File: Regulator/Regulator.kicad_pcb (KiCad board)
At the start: 2 copper layers, 10.2 x 12.7 mm, 10 parts, among them J1 Conn_01x04, U1 LMR16006+FB

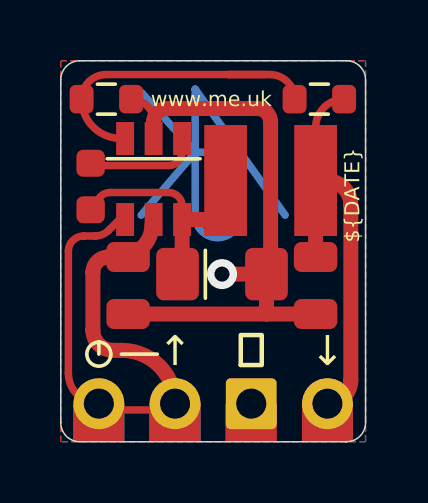
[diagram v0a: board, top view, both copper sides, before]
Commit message: Tweak
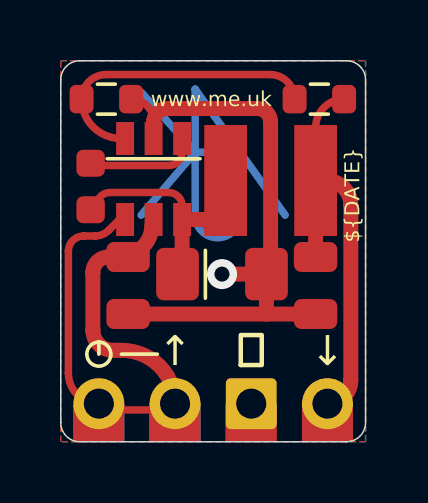
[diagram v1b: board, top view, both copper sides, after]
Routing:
- net Net-(R1-Pad2): track 11.4 -> 10.1 mm
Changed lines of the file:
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@@
   (segment (start 166.33404 62.412) (end 165.9755 62.412) (width 0.5) (layer "F.Cu") (net 2))
   (segment (start 167.15002 69.06998) (end 167.15002 63.22798) (width 0.5) (layer "F.Cu") (net 2))
-  (arc (start 166.1485 61.994342) (mid 166.103539 62.220377) (end 165.9755 62.412) (width 0.5) (layer "F.Cu") (net 2))
   (arc (start 167.15002 63.22798) (mid 166.911025 62.650995) (end 166.33404 62.412) (width 0.5) (layer "F.Cu") (net 2))
   (arc (start 166.925 59.7) (mid 166.253602 59.978102) (end 165.9755 60.6495) (width 0.25) (layer "F.Cu") (net 2))
   (arc (start 166.37 69.85) (mid 166.921557 69.621537) (end 167.15002 69.06998) (width 0.5) (layer "F.Cu") (net 2))
-  (segment (start 164.33398 58.87948) (end 163.07948 58.87948) (width 0.25) (layer "F.Cu") (net 3))
   (segment (start 159.487 61.012) (end 159.6255 61.012) (width 0.25) (layer "F.Cu") (net 3))
-  (segment (start 163.07948 58.87948) (end 158.99552 58.87948) (width 0.25) (layer "F.Cu") (net 3))
-  (segment (start 163.07948 58.87948) (end 164.45448 58.87948) (width 0.25) (layer "F.Cu") (net 3))
+  (segment (start 158.99552 58.87948) (end 164.45448 58.87948) (width 0.25) (layer "F.Cu") (net 3))
   (arc (start 158.175 59.7) (mid 158.559276 60.627724) (end 159.487 61.012) (width 0.25) (layer "F.Cu") (net 3))
   (arc (start 164.45448 58.87948) (mid 165.034675 59.119805) (end 165.275 59.7) (width 0.25) (layer "F.Cu") (net 3))

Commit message: Tweaks
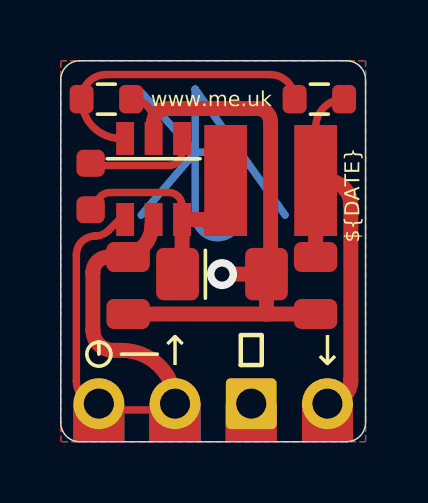
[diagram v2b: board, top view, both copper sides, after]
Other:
- rule pad_to_mask_clearance: 0 -> 0.125
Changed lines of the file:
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@@
       (dielectric_constraints no)
     )
-    (pad_to_mask_clearance 0)
+    (pad_to_mask_clearance 0.125)
     (pad_to_paste_clearance_ratio -0.02)
     (pcbplotparams
@@
     (effects (font (size 1 1) (thickness 0.15)))
   )
-  (segment (start 158.242 64.262) (end 158.626381 64.262) (width 0.25) (layer "F.Cu") (net 1))
   (segment (start 158.55098 67.40175) (end 158.55098 65.47702) (width 0.5) (layer "F.Cu") (net 1))
   (segment (start 159.512 68.072) (end 159.22123 68.072) (width 0.5) (layer "F.Cu") (net 1))
   (segment (start 159.7255 64.962) (end 159.066 64.962) (width 0.5) (layer "F.Cu") (net 1))
   (segment (start 158.75 70.06) (end 161.29 70.06) (width 0.25) (layer "F.Cu") (net 1))
-  (segment (start 159.438007 63.712) (end 159.6255 63.712) (width 0.25) (layer "F.Cu") (net 1))
-  (segment (start 157.734 68.834) (end 157.734 64.77) (width 0.25) (layer "F.Cu") (net 1))
-  (segment (start 159.073003 64.077003) (end 159.438007 63.712) (width 0.25) (layer "F.Cu") (net 1))
-  (arc (start 158.626381 64.262) (mid 158.868091 64.21392) (end 159.073003 64.077003) (width 0.25) (layer "F.Cu") (net 1))
+  (segment (start 158 64.888381) (end 158 69.1) (width 0.25) (layer "F.Cu") (net 1))
+  (segment (start 159.6255 63.712) (end 159.438007 63.712) (width 0.25) (layer "F.Cu") (net 1))
+  (segment (start 159.438007 63.712) (end 159.073003 64.077003) (width 0.25) (layer "F.Cu") (net 1))
   (arc (start 159.22123 68.072) (mid 158.747292 67.875688) (end 158.55098 67.40175) (width 0.5) (layer "F.Cu") (net 1))
+  (arc (start 159.073003 64.077003) (mid 158.868091 64.21392) (end 158.626381 64.262) (width 0.25) (layer "F.Cu") (net 1))
   (arc (start 161.29 69.85) (mid 160.769236 68.592764) (end 159.512 68.072) (width 0.5) (layer "F.Cu") (net 1))
   (arc (start 159.066 64.962) (mid 158.701826 65.112846) (end 158.55098 65.47702) (width 0.5) (layer "F.Cu") (net 1))
-  (arc (start 157.734 64.77) (mid 157.88279 64.41079) (end 158.242 64.262) (width 0.25) (layer "F.Cu") (net 1))
-  (arc (start 158.75 69.85) (mid 158.03158 69.55242) (end 157.734 68.834) (width 0.25) (layer "F.Cu") (net 1))
+  (arc (start 158 69.1) (mid 158.21967 69.63033) (end 158.75 69.85) (width 0.25) (layer "F.Cu") (net 1))
+  (arc (start 158.626381 64.262) (mid 158.183463 64.445463) (end 158 64.888381) (width 0.25) (layer "F.Cu") (net 1))
   (segment (start 165.9755 60.6495) (end 165.9755 62.412) (width 0.25) (layer "F.Cu") (net 2))
   (segment (start 166.33404 62.412) (end 165.9755 62.412) (width 0.5) (layer "F.Cu") (net 2))

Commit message: Revised rules
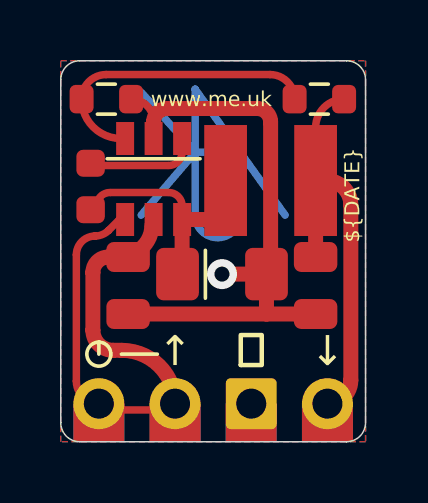
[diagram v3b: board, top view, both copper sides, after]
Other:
- rule pad_to_mask_clearance: 0.125 -> 0.01
